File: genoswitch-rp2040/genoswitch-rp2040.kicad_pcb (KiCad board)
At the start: 2 copper layers, 37 parts, among them J1 USB_B_Micro, J2 Conn_01x03_Socket-PicoDebug, J3 HW-SPI0, J4 HW-SPI1, J5 PIO-SPI0, J6 PIO-SPI1, J7 SERIAL, SW1 PTS815_SJM_250_SMTR_LFS, U1 NCP1117-3.3_SOT223, U2 W25Q128JVS, U3 RP2040, U4 MCP1501-10xCH, Y1 ABLS-12.000MHZ-B4-T

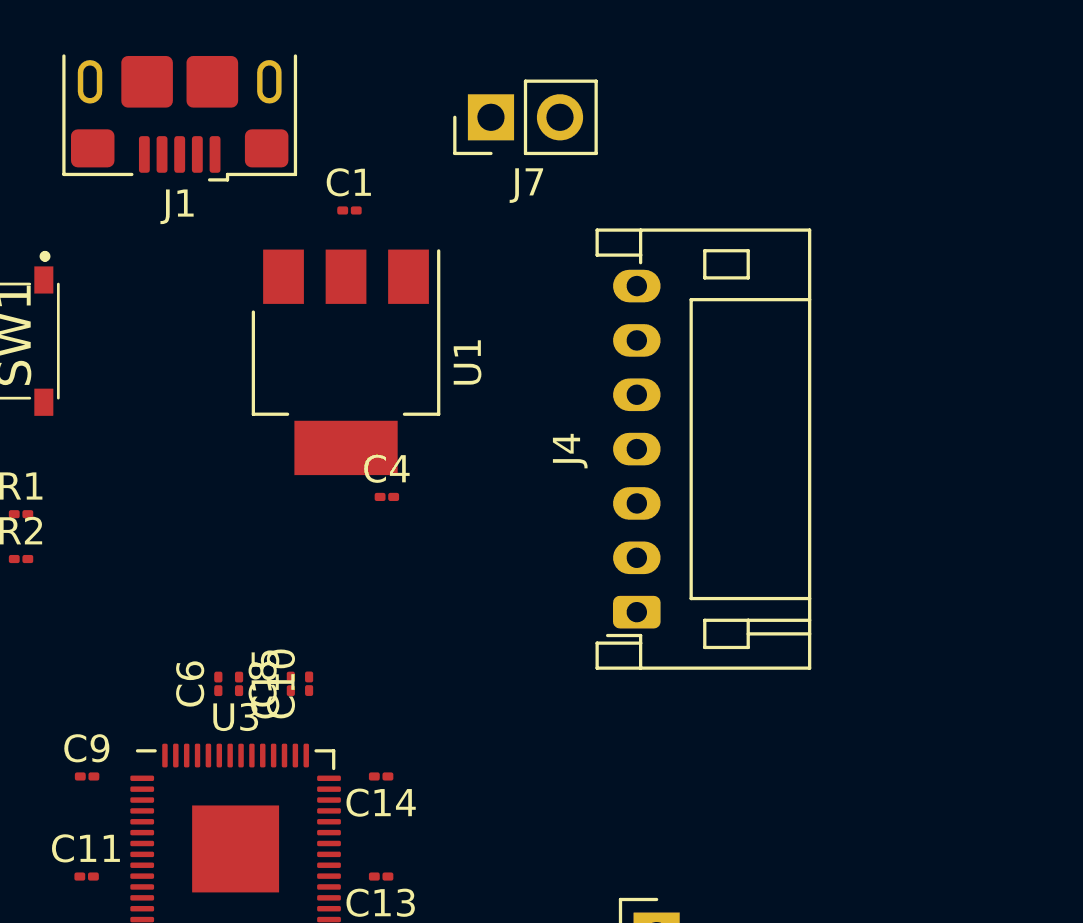
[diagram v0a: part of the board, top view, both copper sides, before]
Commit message: Route USB Data Lines
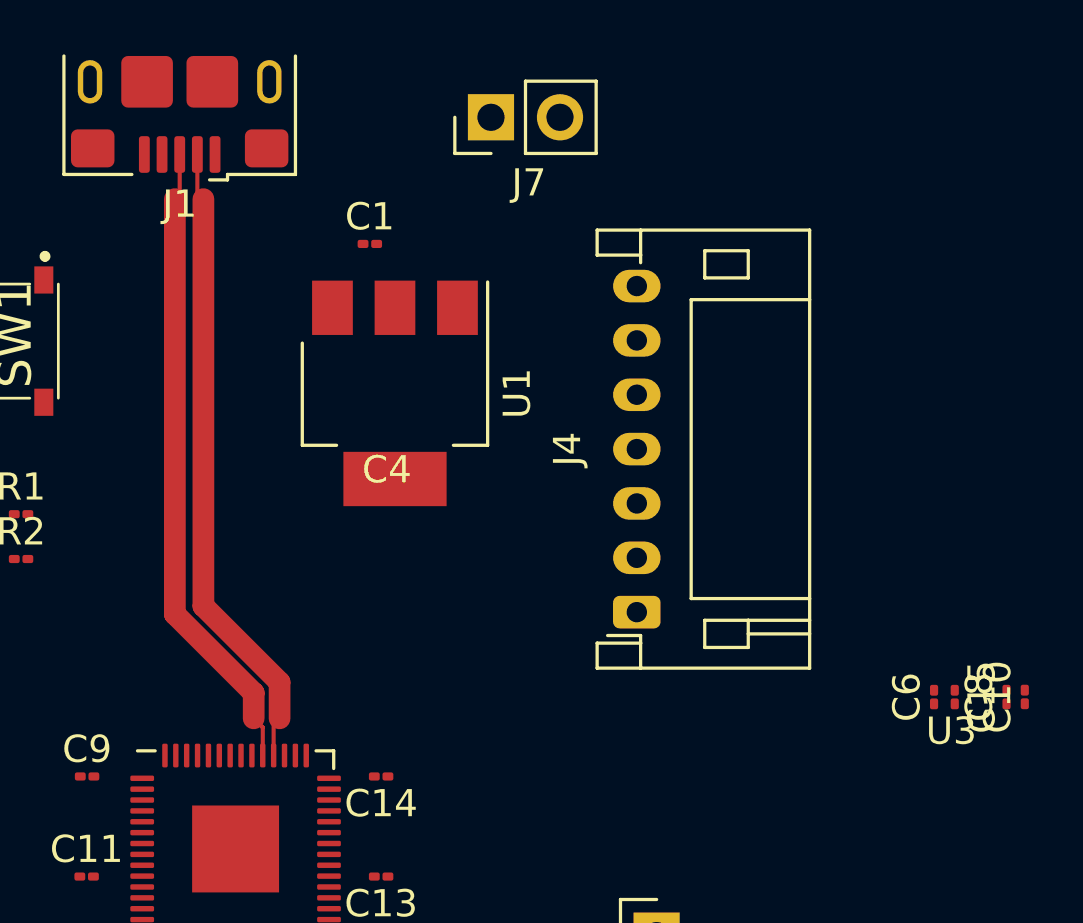
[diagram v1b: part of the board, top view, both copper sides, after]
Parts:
- moved C15 26.3 mm to (135.8, 68.3)
- moved C6 26.3 mm to (135.1, 68.3)
- moved C8 26.3 mm to (137.7, 68.3)
- moved C10 26.3 mm to (138.4, 68.3)
- moved U1 2.13 mm to (115.2, 57.1)
- moved C1 1.44 mm to (114.3, 51.6)
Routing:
- net /USB_D+: track 0.00 -> 23.5 mm
- net /USB_D-: track 0.00 -> 23.5 mm
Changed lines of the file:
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@@
   )
   (footprint "Capacitor_SMD:C_01005_0402Metric" (layer "F.Cu")
-    (at 112.052 67.835 90)
+    (at 138.39 68.321 90)
     (descr "Capacitor SMD 01005 (0402 Metric), square (rectangular) end terminal, IPC_7351 nominal, (Body size source: http://www.vishay.com/docs/20056/crcw01005e3.pdf), generated with kicad-footprint-generator")
     (tags "capacitor")
@@
   )
   (footprint "Capacitor_SMD:C_01005_0402Metric" (layer "F.Cu")
-    (at 108.712 67.839 90)
+    (at 135.05 68.325 90)
     (descr "Capacitor SMD 01005 (0402 Metric), square (rectangular) end terminal, IPC_7351 nominal, (Body size source: http://www.vishay.com/docs/20056/crcw01005e3.pdf), generated with kicad-footprint-generator")
     (tags "capacitor")
@@
   )
   (footprint "Capacitor_SMD:C_01005_0402Metric" (layer "F.Cu")
-    (at 109.474 67.839 -90)
+    (at 135.812 68.325 -90)
     (descr "Capacitor SMD 01005 (0402 Metric), square (rectangular) end terminal, IPC_7351 nominal, (Body size source: http://www.vishay.com/docs/20056/crcw01005e3.pdf), generated with kicad-footprint-generator")
     (tags "capacitor")
@@
   )
   (footprint "Package_TO_SOT_SMD:SOT-223-3_TabPin2" (layer "F.Cu")
-    (at 113.411 56.007 -90)
+    (at 115.212 57.15 -90)
     (descr "module CMS SOT223 4 pins")
     (tags "CMS SOT")
@@
   )
   (footprint "Capacitor_SMD:C_01005_0402Metric" (layer "F.Cu")
-    (at 113.538 50.419)
+    (at 114.287 51.65)
     (descr "Capacitor SMD 01005 (0402 Metric), square (rectangular) end terminal, IPC_7351 nominal, (Body size source: http://www.vishay.com/docs/20056/crcw01005e3.pdf), generated with kicad-footprint-generator")
     (tags "capacitor")
@@
   )
   (footprint "Capacitor_SMD:C_01005_0402Metric" (layer "F.Cu")
-    (at 111.379 67.839 90)
+    (at 137.717 68.325 90)
     (descr "Capacitor SMD 01005 (0402 Metric), square (rectangular) end terminal, IPC_7351 nominal, (Body size source: http://www.vishay.com/docs/20056/crcw01005e3.pdf), generated with kicad-footprint-generator")
     (tags "capacitor")
@@
     (property "ki_keywords" "RP2040 ARM Cortex-M0+ USB")
     (attr smd)
-    (fp_text reference "U3" (at 0 -4.82) (layer "F.SilkS")
+    (fp_text reference "U3" (at 26.338 -4.334) (layer "F.SilkS")
         (effects (font (size 1 1) (thickness 0.15)))
     )
@@
     (stroke (width 0.15) (type default)) (layer "User.1"))
   (segment (start 111.544 70.4735) (end 111.547 70.4765) (width 0.15) (layer "F.Cu") (net 7))
+  (segment (start 108.162 50) (end 108.162 64.97655) (width 0.8) (layer "F.Cu") (net 10))
+  (segment (start 107.94 48.358) (end 107.94 49.778) (width 0.1524) (layer "F.Cu") (net 10))
+  (segment (start 108.162 64.97655) (end 110.965231 67.779781) (width 0.8) (layer "F.Cu") (net 10))
+  (segment (start 107.94 49.778) (end 108.162 50) (width 0.1524) (layer "F.Cu") (net 10))
+  (segment (start 110.747 70.4765) (end 110.747 69.326447) (width 0.1524) (layer "F.Cu") (net 10))
+  (segment (start 110.965231 67.779781) (end 110.965231 69.108216) (width 0.8) (layer "F.Cu") (net 10))
+  (segment (start 110.747 69.326447) (end 110.965231 69.108216) (width 0.1524) (layer "F.Cu") (net 10))
+  (segment (start 110.347 70.4765) (end 110.347 69.442385) (width 0.1524) (layer "F.Cu") (net 11))
+  (segment (start 110.347 69.442385) (end 110.012831 69.108216) (width 0.1524) (layer "F.Cu") (net 11))
+  (segment (start 107.112 65.27345) (end 110.012831 68.174281) (width 0.8) (layer "F.Cu") (net 11))
+  (segment (start 110.012831 68.174281) (end 110.012831 69.108216) (width 0.8) (layer "F.Cu") (net 11))
+  (segment (start 107.112 50) (end 107.112 65.27345) (width 0.8) (layer "F.Cu") (net 11))
+  (segment (start 107.29 48.358) (end 107.29 49.822) (width 0.1524) (layer "F.Cu") (net 11))
+  (segment (start 107.29 49.822) (end 107.112 50) (width 0.1524) (layer "F.Cu") (net 11))
 )
